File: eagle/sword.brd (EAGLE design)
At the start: 14.9 x 24.1 mm, 4 parts, among them U1 TINY45-20-DIP

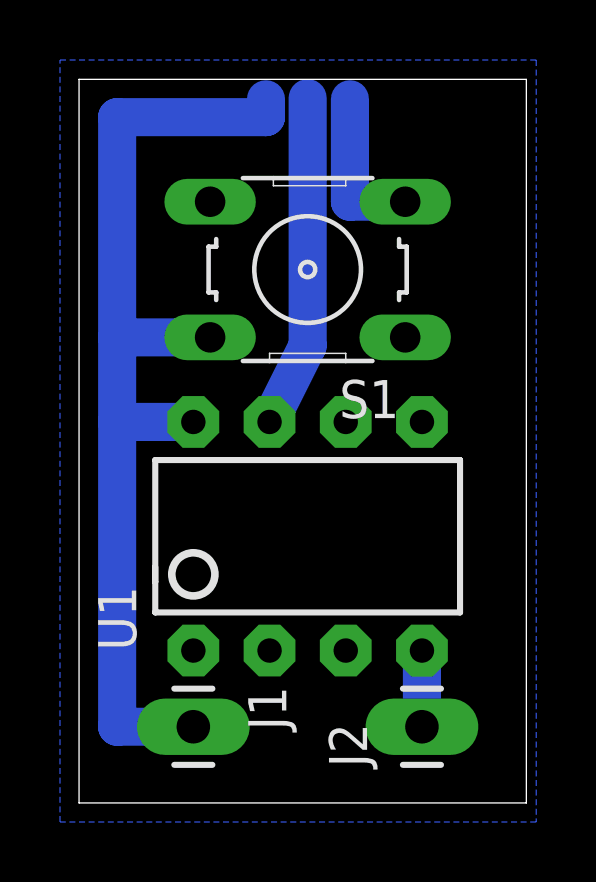
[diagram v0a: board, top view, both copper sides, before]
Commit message: major schematic fail...
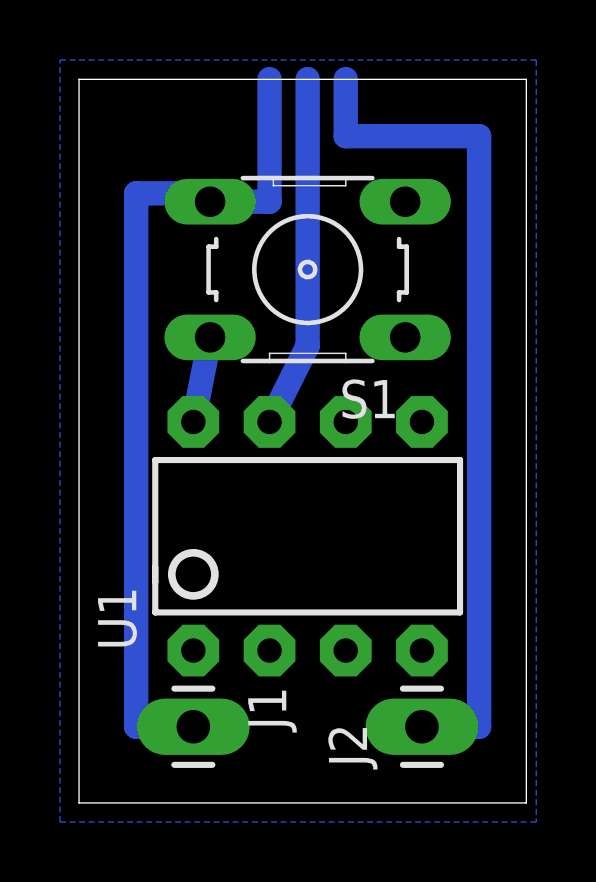
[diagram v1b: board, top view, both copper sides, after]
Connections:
- new net N$1: J1.1, S1.4
- net GND: no longer S1.3
- net VCC: no longer J1.1
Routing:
- net VCC: track 34.1 -> 2.87 mm
- net N$1: track 0.00 -> 28.5 mm
- net GND: track 7.80 -> 27.9 mm
- net DIN: track 11.1 -> 11.7 mm
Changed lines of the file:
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@@
 <?xml version="1.0" encoding="utf-8"?>
 <!DOCTYPE eagle SYSTEM "eagle.dtd">
-<eagle version="7.5.0">
+<eagle version="8.0.0">
 <drawing>
 <settings>
@@
 <setting verticaltext="up"/>
 </settings>
-<grid distance="0.0001" unitdist="inch" unit="inch" style="lines" multiple="1" display="no" altdistance="0.025" altunitdist="inch" altunit="inch"/>
+<grid distance="0.025" unitdist="inch" unit="inch" style="lines" multiple="1" display="no" altdistance="0.025" altunitdist="inch" altunit="inch"/>
 <layers>
 <layer number="1" name="Top" color="4" fill="1" visible="yes" active="yes"/>
@@
 <contactref element="U1" pad="8"/>
 <contactref element="S1" pad="2"/>
-<contactref element="J1" pad="1"/>
-<wire x1="3.81" y1="2.54" x2="1.27" y2="2.54" width="1.27" layer="16"/>
-<wire x1="1.27" y1="2.54" x2="1.27" y2="12.7" width="1.27" layer="16"/>
-<wire x1="1.27" y1="12.7" x2="3.81" y2="12.7" width="1.27" layer="16"/>
-<wire x1="1.27" y1="15.5194" x2="1.27" y2="22.86" width="1.27" layer="16"/>
-<wire x1="1.27" y1="22.86" x2="6.23061875" y2="22.86" width="1.27" layer="16"/>
-<wire x1="4.3688" y1="15.5194" x2="1.27" y2="15.5194" width="1.27" layer="16"/>
-<wire x1="1.27" y1="12.7" x2="1.27" y2="15.5194" width="1.27" layer="16"/>
-<wire x1="6.23061875" y1="22.86" x2="6.23061875" y2="23.4569" width="1.27" layer="16"/>
-<wire x1="6.23061875" y1="23.4569" x2="6.1976" y2="24.13" width="0" layer="19" extent="1-16"/>
+<wire x1="3.81" y1="12.7" x2="4.3688" y2="15.5194" width="0.8128" layer="16"/>
 </signal>
 <signal name="GND">
 <contactref element="U1" pad="4"/>
-<contactref element="S1" pad="3"/>
 <contactref element="J2" pad="1"/>
-<wire x1="11.43" y1="5.08" x2="11.43" y2="2.54" width="1.27" layer="16"/>
 <polygon width="1.27" layer="16" thermals="no">
 <vertex x="0" y="24.765"/>
@@
 <vertex x="-0.635" y="24.765"/>
 </polygon>
-<wire x1="10.8712" y1="20.0406" x2="9.0297" y2="20.0406" width="1.27" layer="16"/>
-<wire x1="9.0297" y1="20.0406" x2="9.0297" y2="23.4569" width="1.27" layer="16"/>
-<wire x1="9.0297" y1="23.4569" x2="9.0424" y2="24.13" width="0" layer="19" extent="1-16"/>
+<wire x1="11.43" y1="2.54" x2="13.335" y2="2.54" width="0.8128" layer="16"/>
+<wire x1="13.335" y1="2.54" x2="13.335" y2="22.225" width="0.8128" layer="16"/>
+<wire x1="13.335" y1="22.225" x2="8.89" y2="22.225" width="0.8128" layer="16"/>
+<wire x1="8.89" y1="22.225" x2="8.89" y2="24.13" width="0.8128" layer="16"/>
 </signal>
 <signal name="DIN">
 <contactref element="U1" pad="7"/>
-<wire x1="6.35" y1="12.7" x2="7.62" y2="15.24" width="1.27" layer="16"/>
-<wire x1="7.62" y1="15.24" x2="7.62" y2="23.495" width="1.27" layer="16"/>
-<wire x1="7.62" y1="23.495" x2="7.62" y2="24.13" width="0" layer="19" extent="1-16"/>
+<wire x1="6.35" y1="12.7" x2="7.62" y2="15.24" width="0.8128" layer="16"/>
+<wire x1="7.62" y1="15.24" x2="7.62" y2="24.13" width="0.8128" layer="16"/>
+</signal>
+<signal name="N$1">
+<contactref element="J1" pad="1"/>
+<contactref element="S1" pad="4"/>
+<wire x1="3.81" y1="2.54" x2="1.905" y2="2.54" width="0.8128" layer="16"/>
+<wire x1="1.905" y1="2.54" x2="1.905" y2="20.32" width="0.8128" layer="16"/>
+<wire x1="1.905" y1="20.32" x2="4.3688" y2="20.32" width="0.8128" layer="16"/>
+<wire x1="4.3688" y1="20.32" x2="4.3688" y2="20.0406" width="0.8128" layer="16"/>
+<wire x1="4.3688" y1="20.0406" x2="6.35" y2="20.0406" width="0.8128" layer="16"/>
+<wire x1="6.35" y1="20.0406" x2="6.35" y2="24.13" width="0.8128" layer="16"/>
 </signal>
 </signals>
